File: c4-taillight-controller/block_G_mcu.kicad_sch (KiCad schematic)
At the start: 7 parts, among them U1 nRF52840, X1 32MHz

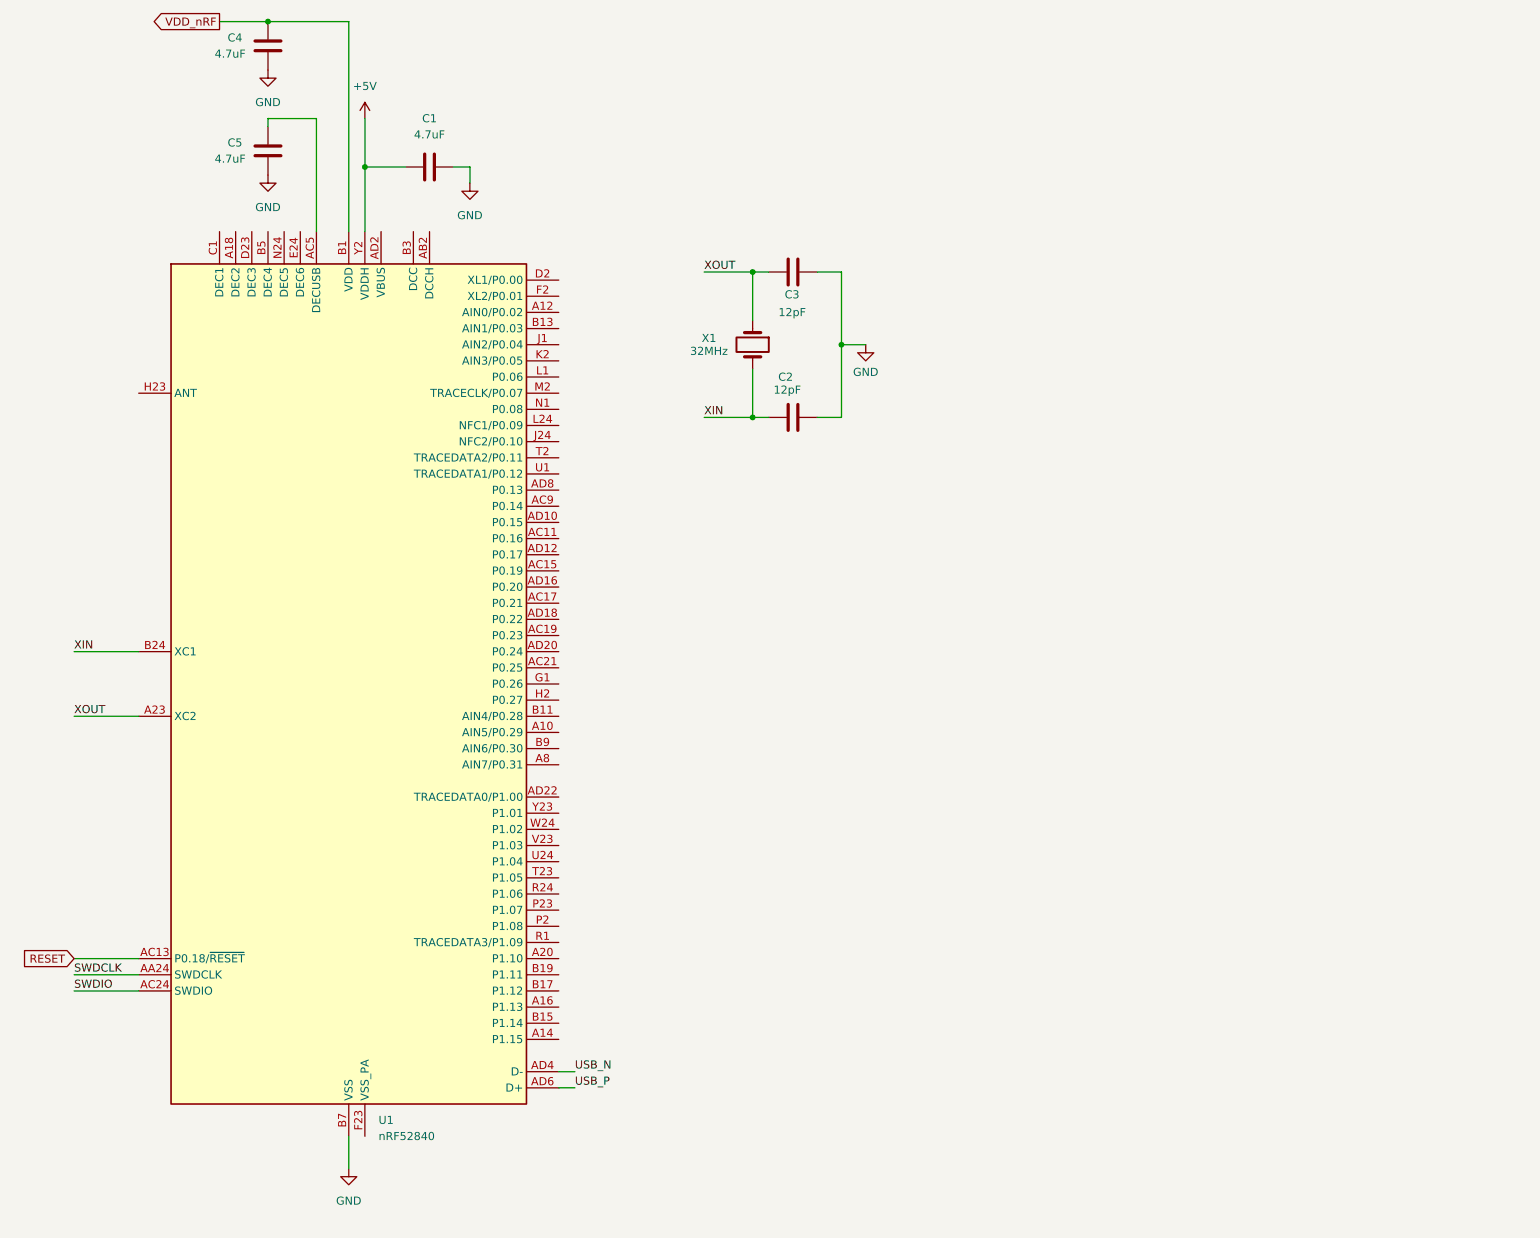
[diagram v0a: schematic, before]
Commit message: bare-si nrF52840
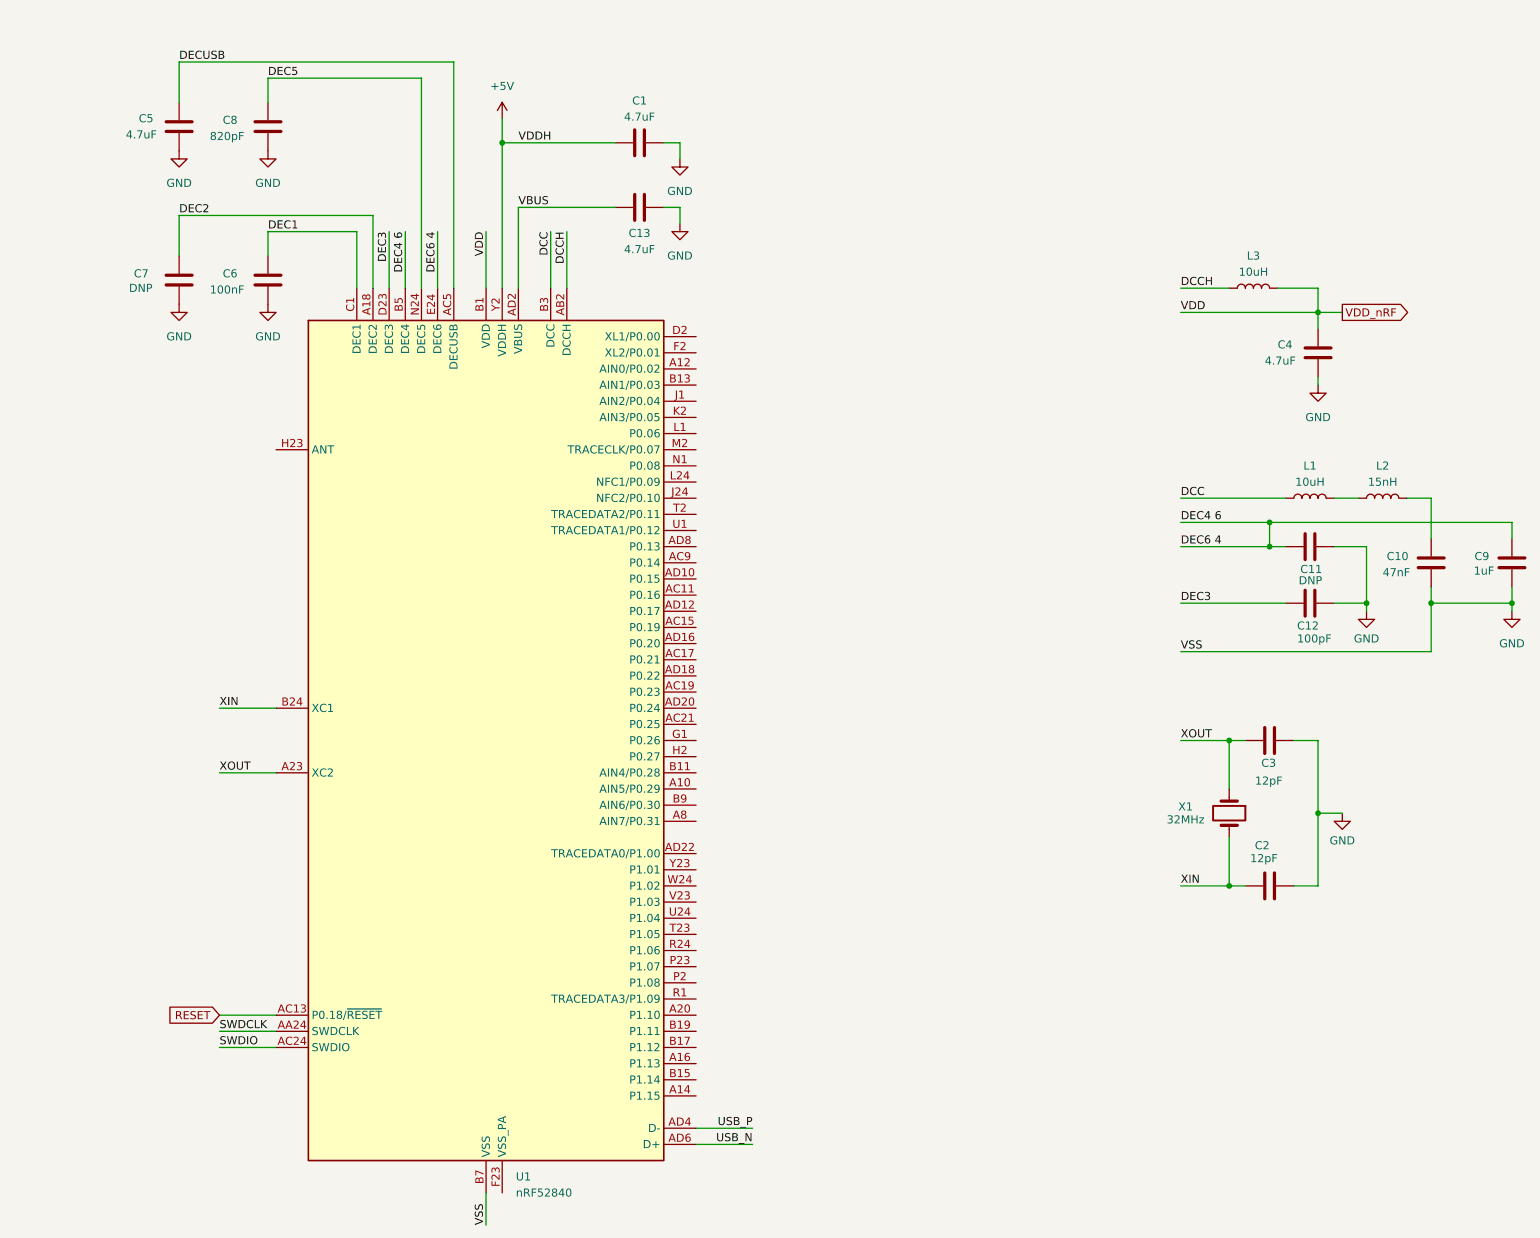
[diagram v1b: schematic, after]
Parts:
- added C10: 47nF, symbol Device:C
- added C11, C7: DNP, symbol Device:C
- added C12: 100pF, symbol Device:C
- added C13: 4.7uF, symbol Device:C
- added C6: 100nF, symbol Device:C
- added C8: 820pF, symbol Device:C
- added C9: 1uF, symbol Device:C
- added L1, L3: 10uH, symbol Device:L
- added L2: 15nH, symbol Device:L
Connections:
- net GND: now also C10.1, C11.1, C12.1, C13.1, C6.2, C7.2, C8.2, C9.1
- net USB_N: now also U1.AD6 (D+); no longer U1.AD4 (D-)
- net USB_P: now also U1.AD4 (D-); no longer U1.AD6 (D+)
- net VDD_nRF: now also L3.2
- net DEC2: now reaches U1.A18 (DEC2)
- net DEC2: now also C7.1
- net DCCH: now reaches U1.AB2 (DCCH)
- net DCCH: now also L3.1
- net DECUSB: now reaches C5.1, U1.AC5 (DECUSB)
- net VBUS: now reaches U1.AD2 (VBUS)
- net VBUS: now also C13.2
- net DCC: now reaches U1.B3 (DCC)
- net DCC: now also L1.1
- net DEC4 6: now reaches U1.B5 (DEC4)
- net DEC4 6: now also U1.E24 (DEC6), C11.2, C9.2
- net DEC1: now reaches U1.C1 (DEC1)
- net DEC1: now also C6.1
- net DEC3: now reaches U1.D23 (DEC3)
- net DEC3: now also C12.2
- net DEC5: now reaches U1.N24 (DEC5)
- net DEC5: now also C8.1
- new net: L1.2, L2.1
- new net: C10.2, L2.2
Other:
- moved on the sheet: C1, C2, C3, C4, C5, U1, X1
